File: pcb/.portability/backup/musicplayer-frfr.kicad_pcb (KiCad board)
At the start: 2 copper layers, 61.2 x 78.2 mm, 23 parts, among them J1 Battery, J2 AudioPlug3, J3 Display, SW1 SW_Push, SW2 SW_Push, SW3 SW_Push, SW4 RotaryEncoder_Switch, SW5 SW_SPDT, U1 XIAO-RP2350-SMD, U2 TP4056-42-ESOP8, U3 DFPLAYER_MINI

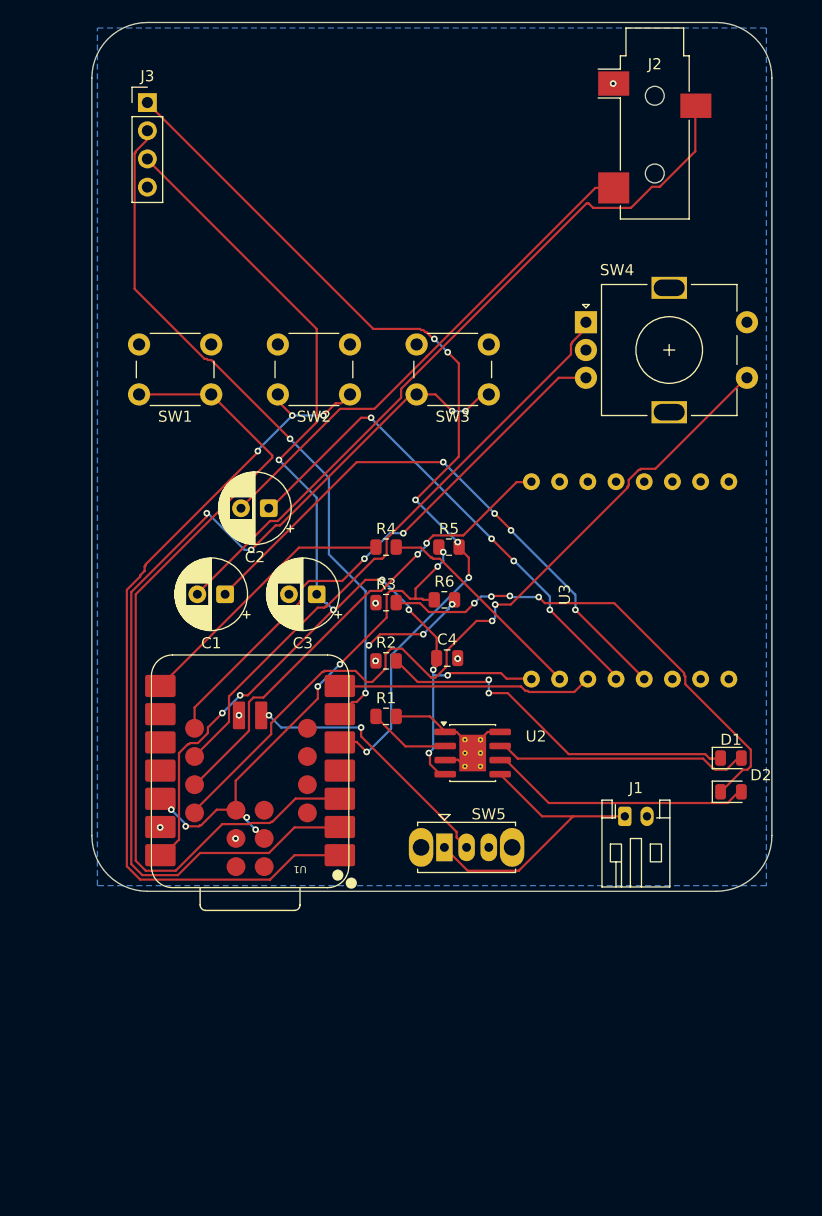
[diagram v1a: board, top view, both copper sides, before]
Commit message: Generated PCB production files
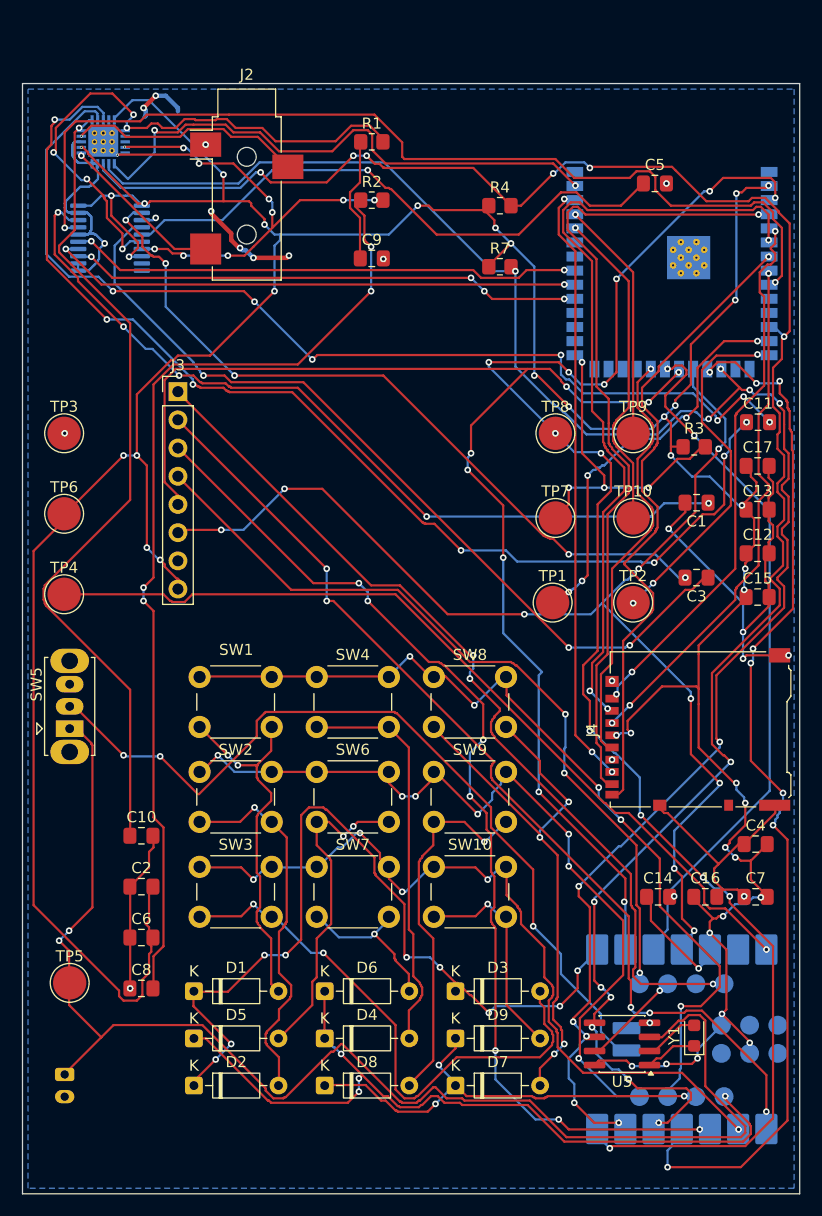
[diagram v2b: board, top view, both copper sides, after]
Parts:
- removed R5, R6: 4.7k, Resistor_SMD:R_0805_2012Metric
- added C10: 1uF, Capacitor_SMD:C_0805_2012Metric_Pad1.18x1.45mm_HandSolder, F.Cu at (110.7, 107.8)
- added C11: 1uF, Capacitor_SMD:C_0805_2012Metric_Pad1.18x1.45mm_HandSolder, F.Cu at (166.2, 70.5)
- added C12: 1uF, Capacitor_SMD:C_0805_2012Metric_Pad1.18x1.45mm_HandSolder, F.Cu at (166.2, 82.3)
- added C13: 0.1u, Capacitor_SMD:C_0805_2012Metric_Pad1.18x1.45mm_HandSolder, F.Cu at (166.2, 78.4)
- added C14: 10u, Capacitor_SMD:C_0805_2012Metric_Pad1.18x1.45mm_HandSolder, F.Cu at (157.2, 113.2)
- added C15: 10u, Capacitor_SMD:C_0805_2012Metric_Pad1.18x1.45mm_HandSolder, F.Cu at (166.2, 86.2)
- added C16: 10u, Capacitor_SMD:C_0805_2012Metric_Pad1.18x1.45mm_HandSolder, F.Cu at (161.5, 113.2)
- added C17: 10u, Capacitor_SMD:C_0805_2012Metric_Pad1.18x1.45mm_HandSolder, F.Cu at (166.2, 74.4)
- added C5: 2.2uF, Capacitor_SMD:C_0805_2012Metric_Pad1.18x1.45mm_HandSolder, F.Cu at (157.0, 49.0)
- added C6: 100nF, Capacitor_SMD:C_0805_2012Metric_Pad1.18x1.45mm_HandSolder, F.Cu at (110.7, 116.9)
- added C7: 10uF, Capacitor_SMD:C_0805_2012Metric_Pad1.18x1.45mm_HandSolder, F.Cu at (166.0, 113.2)
- added C8: 2.2nF, Capacitor_SMD:C_0805_2012Metric_Pad1.18x1.45mm_HandSolder, F.Cu at (110.7, 121.5)
- added C9: 2.2nF, Capacitor_SMD:C_0805_2012Metric_Pad1.18x1.45mm_HandSolder, F.Cu at (131.5, 55.8)
- added D3: 1N4149, Diode_THT:D_DO-35_SOD27_P7.62mm_Horizontal, F.Cu at (139.0, 121.8)
- added D4: 1N4149, Diode_THT:D_DO-35_SOD27_P7.62mm_Horizontal, F.Cu at (127.2, 126.0)
- added D5: 1N4149, Diode_THT:D_DO-35_SOD27_P7.62mm_Horizontal, F.Cu at (115.4, 126.0)
- added D6: 1N4149, Diode_THT:D_DO-35_SOD27_P7.62mm_Horizontal, F.Cu at (127.2, 121.8)
- added D7: 1N4149, Diode_THT:D_DO-35_SOD27_P7.62mm_Horizontal, F.Cu at (139.0, 130.2)
- added D8: 1N4149, Diode_THT:D_DO-35_SOD27_P7.62mm_Horizontal, F.Cu at (127.2, 130.2)
- added D9: 1N4149, Diode_THT:D_DO-35_SOD27_P7.62mm_Horizontal, F.Cu at (139.0, 126.0)
- added J4: Micro_SD_Card_Det1, Connector_Card:microSD_HC_Hirose_DM3AT-SF-PEJM5, F.Cu at (160.8, 98.2)
- added R7: 4.7k, Resistor_SMD:R_0805_2012Metric_Pad1.20x1.40mm_HandSolder, F.Cu at (143.0, 56.5)
- added SW10: Next, Button_Switch_THT:SW_PUSH_6mm, F.Cu at (137.1, 110.5)
- added SW6: Select, Button_Switch_THT:SW_PUSH_6mm, F.Cu at (126.5, 102.0)
- added SW7: Right, Button_Switch_THT:SW_PUSH_6mm, F.Cu at (126.5, 110.5)
- added SW8: Prev., Button_Switch_THT:SW_PUSH_6mm, F.Cu at (137.1, 93.5)
- added SW9: Down, Button_Switch_THT:SW_PUSH_6mm, F.Cu at (137.1, 102.0)
- added TP1: USB D-, TestPoint:TestPoint_Pad_D3.0mm, F.Cu at (147.8, 86.8)
- added TP10: ESP RX, TestPoint:TestPoint_Pad_D3.0mm, F.Cu at (155.0, 79.1)
- added TP2: USB D+, TestPoint:TestPoint_Pad_D3.0mm, F.Cu at (155.0, 86.8)
- added TP3: GND, TestPoint:TestPoint_Pad_D3.0mm, F.Cu at (103.8, 71.5)
- added TP4: +5V, TestPoint:TestPoint_Pad_D3.0mm, F.Cu at (103.8, 86.0)
- added TP5: VBAT, TestPoint:TestPoint_Pad_D3.0mm, F.Cu at (104.2, 121.0)
- added TP6: +3V3, TestPoint:TestPoint_Pad_D3.0mm, F.Cu at (103.8, 78.8)
- added TP7: ESP Boot, TestPoint:TestPoint_Pad_D3.0mm, F.Cu at (148.0, 79.1)
- added TP8: ESP Enable, TestPoint:TestPoint_Pad_D3.0mm, F.Cu at (148.0, 71.5)
- added TP9: ESP TX, TestPoint:TestPoint_Pad_D3.0mm, F.Cu at (155.0, 71.5)
- added U4: ESP32-S3-WROOM-1, RF_Module:ESP32-S3-WROOM-1, B.Cu at (158.5, 53.2)
- added U5: PCF8523T, Package_SO:SOIC-8_3.9x4.9mm_P1.27mm, F.Cu at (154.0, 126.5)
- added Y1: 32.768 kHz, Crystal:Crystal_SMD_2012-2Pin_2.0x1.2mm_HandSoldering, F.Cu at (160.5, 125.8)
- C1, C2: value 100u -> 100nF; footprint Capacitor_THT:CP_Radial_D6.3mm_P2.50mm -> Capacitor_SMD:C_0805_2012Metric_Pad1.18x1.45mm_HandSolder
- C3: value 100u -> 2.2uF; footprint Capacitor_THT:CP_Radial_D6.3mm_P2.50mm -> Capacitor_SMD:C_0805_2012Metric_Pad1.18x1.45mm_HandSolder
- C4: value 0.1u -> 100nF; footprint Capacitor_SMD:C_0805_2012Metric -> Capacitor_SMD:C_0805_2012Metric_Pad1.18x1.45mm_HandSolder
- D1, D2: value LED -> 1N4149; footprint LED_SMD:LED_0805_2012Metric -> Diode_THT:D_DO-35_SOD27_P7.62mm_Horizontal
- J1, U1: moved to B.Cu
- J3: footprint Connector_PinHeader_2.54mm:PinHeader_1x04_P2.54mm_Vertical -> Connector_PinHeader_2.54mm:PinHeader_1x08_P2.54mm_Vertical
- R1: value 2.4K -> 470; footprint Resistor_SMD:R_0805_2012Metric -> Resistor_SMD:R_0805_2012Metric_Pad1.20x1.40mm_HandSolder
- R2: value 1K -> 470; footprint Resistor_SMD:R_0805_2012Metric -> Resistor_SMD:R_0805_2012Metric_Pad1.20x1.40mm_HandSolder
- R3: value 1K -> 10k; footprint Resistor_SMD:R_0805_2012Metric -> Resistor_SMD:R_0805_2012Metric_Pad1.20x1.40mm_HandSolder
- R4: value 1K -> 4.7k; footprint Resistor_SMD:R_0805_2012Metric -> Resistor_SMD:R_0805_2012Metric_Pad1.20x1.40mm_HandSolder
- SW1: value SW_Push -> Vol Up
- SW2: value SW_Push -> Up
- SW3: value SW_Push -> Vol Down
- SW4: value RotaryEncoder_Switch -> Left; footprint Rotary_Encoder:RotaryEncoder_Alps_EC11E-Switch_Vertical_H20mm -> Button_Switch_THT:SW_PUSH_6mm
- SW5: value SW_SPDT -> SW_BAT
- U2: value TP4056-42-ESOP8 -> TPA6130A2RTJT; footprint Package_SO:SOIC-8-1EP_3.9x4.9mm_P1.27mm_EP2.41x3.3mm_ThermalVias -> footprints:RTJ20_2P7X2P7; moved to B.Cu
- U3: value DFPLAYER_MINI -> PCM5102; footprint DFPlayer:DFPlayer_V2 -> Package_SO:TSSOP-20_4.4x6.5mm_P0.65mm; moved to B.Cu
- moved U2 64.3 mm to (107.3, 45.2), turned to 180 degrees
- moved J1 55.5 mm to (103.8, 129.2), turned to -90 degrees
- moved D2 55.1 mm to (115.4, 130.2)
- moved D1 52.7 mm to (115.4, 121.8)
- moved R1 51.8 mm to (131.5, 45.2)
- moved SW3 49.9 mm to (116.0, 110.5), turned to 0 degrees
- moved U3 49.7 mm to (107.9, 53.9), turned to 180 degrees
- moved U1 45.8 mm to (159.4, 126.1), turned to 0 degrees
- moved C1 43.3 mm to (160.7, 77.8)
- moved R2 41.5 mm to (131.5, 50.5)
- moved SW4 40.1 mm to (126.5, 93.5)
- moved J2 37.2 mm to (120.2, 49.1)
- moved SW2 36.6 mm to (116.0, 102.0), turned to 0 degrees
- moved C2 36.0 mm to (110.7, 112.3), turned to 0 degrees
- moved SW5 35.4 mm to (104.2, 98.1), turned to 90 degrees
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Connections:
- net /NEXT renamed /COL3
- C1 pad 1: Net-(U3-DAC_L) -> Net-(U3-LDOO)
- C1 pad 2: /LEFT -> GND
- C2 pad 1: Net-(U3-DAC_R) -> GND
- C2 pad 2: /RIGHT -> +3V3
- C3 pad 1: /VBUS -> Net-(U3-CAPM)
- C3 pad 2: GND -> Net-(U3-CAPP)
- C4 pad 1: /VBUS -> GND
- C4 pad 2: GND -> +3V3
- D1 pad 1: Net-(D1-K) -> /ROW1
- D1 pad 2: /CHRG -> Net-(D1-A)
- D2 pad 1: Net-(D2-K) -> /ROW1
- D2 pad 2: /STDBY -> Net-(D2-A)
- J2 pad R: /LEFT -> /Audio/HPLEFT
- J2 pad T: /RIGHT -> /Audio/HPRIGHT
- J3 pad 1: /SDA -> /DISPLAY_LIGHT
- J3 pad 2: /SCL -> /DISPLAY_RST
- J3 pad 3: /VBUS -> /DISPLAY_DC
- J3 pad 4: GND -> /DISPLAY_CS
- R1 pad 1: Net-(U2-PROG) -> Net-(C9-Pad1)
- R1 pad 2: GND -> /Audio/OUTL
- R2 pad 1: GND -> Net-(C8-Pad2)
- R2 pad 2: Net-(D1-K) -> /Audio/OUTR
- R3 pad 1: GND -> +3V3
- R3 pad 2: Net-(D2-K) -> /ESP_BOOT
- R4 pad 1: /XIAO_TX -> +3V3
- R4 pad 2: Net-(U3-RX) -> /SDA
- SW1 pad 1: /BACK -> /COL1
- SW1 pad 2: GND -> Net-(D1-A)
- SW2 pad 1: /PLAY -> /COL2
- SW2 pad 2: GND -> Net-(D2-A)
- SW3 pad 2: GND -> Net-(D3-A)
- U1 pad 1: /PLAY -> /DISPLAY_RST
- U1 pad 10: unconnected-(U1-D9-Pad10) -> /SPI_MISO
- U1 pad 11: unconnected-(U1-D10-Pad11) -> /SPI_MOSI
- U1 pad 14: /VBUS -> +5V
- U1 pad 15: /ENCODER_SWITCH -> /DISPLAY_LIGHT
- U1 pad 16: /BUSY -> unconnected-(U1-D12-Pad16)
- U1 pad 17: /ENCODER_A -> /INTA
- U1 pad 18: /ENCODER_B -> /DISPLAY_CS
- U1 pad 19: unconnected-(U1-D15-Pad19) -> /COL2
- U1 pad 20: unconnected-(U1-D16-Pad20) -> /COL1
- U1 pad 21: unconnected-(U1-D17-Pad21) -> /ROW3
- U1 pad 22: unconnected-(U1-D18-Pad22) -> /ROW2
- U1 pad 3: /BACK -> /DISPLAY_DC
- U1 pad 4: unconnected-(U1-D3-Pad4) -> /SPI_CS
- U1 pad 7: /XIAO_RX -> /ESP_ENABLE
- U1 pad 8: /XIAO_TX -> /ROW1
- U1 pad 9: unconnected-(U1-D8-Pad9) -> /SPI_SCK
- U2 pad 1: GND -> /Audio/OUTL
- U2 pad 2: Net-(U2-PROG) -> GND
- U2 pad 4: /VBUS -> /Audio/OUTR
- U2 pad 5: /VBAT -> GND
- U2 pad 6: /STDBY -> /AMP_SDN
- U2 pad 7: /CHRG -> /SCL
- U2 pad 8: GND -> /SDA
- U3 pad 1: /VBUS -> +3V3
- U3 pad 11: unconnected-(U3-IO_2-Pad11) -> GND
- U3 pad 12: unconnected-(U3-ADKEY_1-Pad12) -> GND
- U3 pad 13: unconnected-(U3-ADKEY_2-Pad13) -> /I2S_BCK
- U3 pad 14: unconnected-(U3-USB+-Pad14) -> /I2S_DIN
- U3 pad 15: unconnected-(U3-USB--Pad15) -> /I2S_LRCK
- U3 pad 16: /BUSY -> GND
- U3 pad 2: Net-(U3-RX) -> Net-(U3-CAPP)
- U3 pad 3: /XIAO_RX -> GND
- U3 pad 4: Net-(U3-DAC_R) -> Net-(U3-CAPM)
- U3 pad 5: Net-(U3-DAC_L) -> /Audio/VNEG
- U3 pad 6: unconnected-(U3-SPK_1-Pad6) -> /Audio/OUTL
- U3 pad 7: GND -> /Audio/OUTR
- U3 pad 8: unconnected-(U3-SPK_2-Pad8) -> +3V3
- U3 pad 9: unconnected-(U3-IO_1-Pad9) -> GND
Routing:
- net +3V3: track 48.2 -> 365.7 mm, vias 8 -> 40
- net /ESP_ENABLE: track 0.00 -> 142.0 mm, vias 0 -> 13
- net /SPI_SCK: track 0.00 -> 121.7 mm, vias 0 -> 8
- net /VBUS: track 115.5 -> 0.00 mm, vias 9 -> 0
- net GND: track 11.9 -> 124.3 mm, vias 7 -> 23
- net /SPI_MOSI: track 0.00 -> 110.3 mm, vias 0 -> 9
- net Net-(U2-CPP): track 0.00 -> 101.6 mm, vias 0 -> 7
- net /SPI_CS: track 0.00 -> 95.2 mm, vias 0 -> 8
- net /VBAT: track 27.3 -> 122.4 mm, vias 0 -> 2
- net /DISPLAY_DC: track 0.00 -> 94.2 mm, vias 0 -> 7
- net /SDA: track 82.8 -> 175.7 mm, vias 6 -> 13
- net /SCL: track 71.8 -> 164.7 mm, vias 5 -> 11
- net Net-(U2-CPN): track 0.00 -> 90.7 mm, vias 0 -> 7
- net /DISPLAY_RST: track 0.00 -> 90.3 mm, vias 0 -> 5
- net Net-(C8-Pad2): track 0.00 -> 88.0 mm, vias 0 -> 4
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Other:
- board size 61.2 x 78.2 mm -> 70 x 100 mm
- board text removed: "DISPLAY GOES HERE"
